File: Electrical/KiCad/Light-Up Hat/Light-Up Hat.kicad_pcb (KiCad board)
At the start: 2 copper layers, 39.9 x 20.1 mm, 18 parts, among them J1 Conn_01x04, Q1 MMBT3906, SW1 SW_SPST, U1 AP1117-33, U2 PIC10F220-IOT

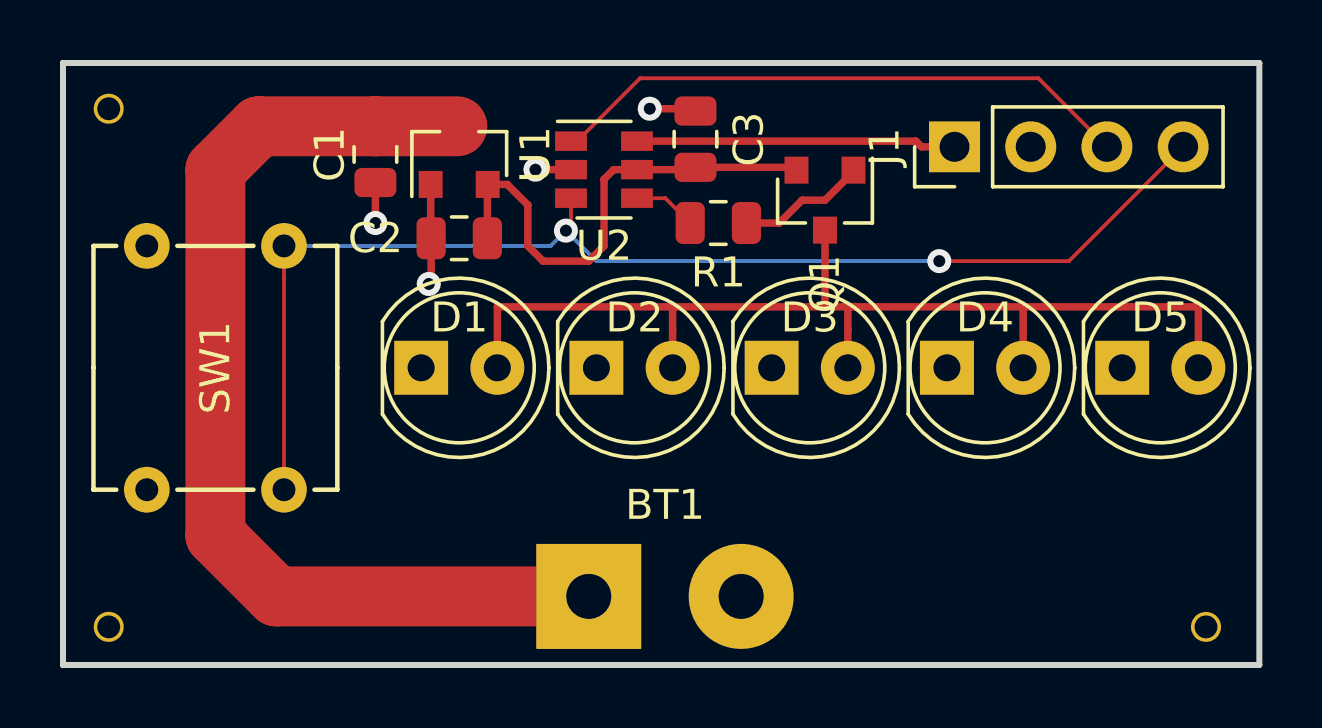
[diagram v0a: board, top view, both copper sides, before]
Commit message: fixed board design for new revision
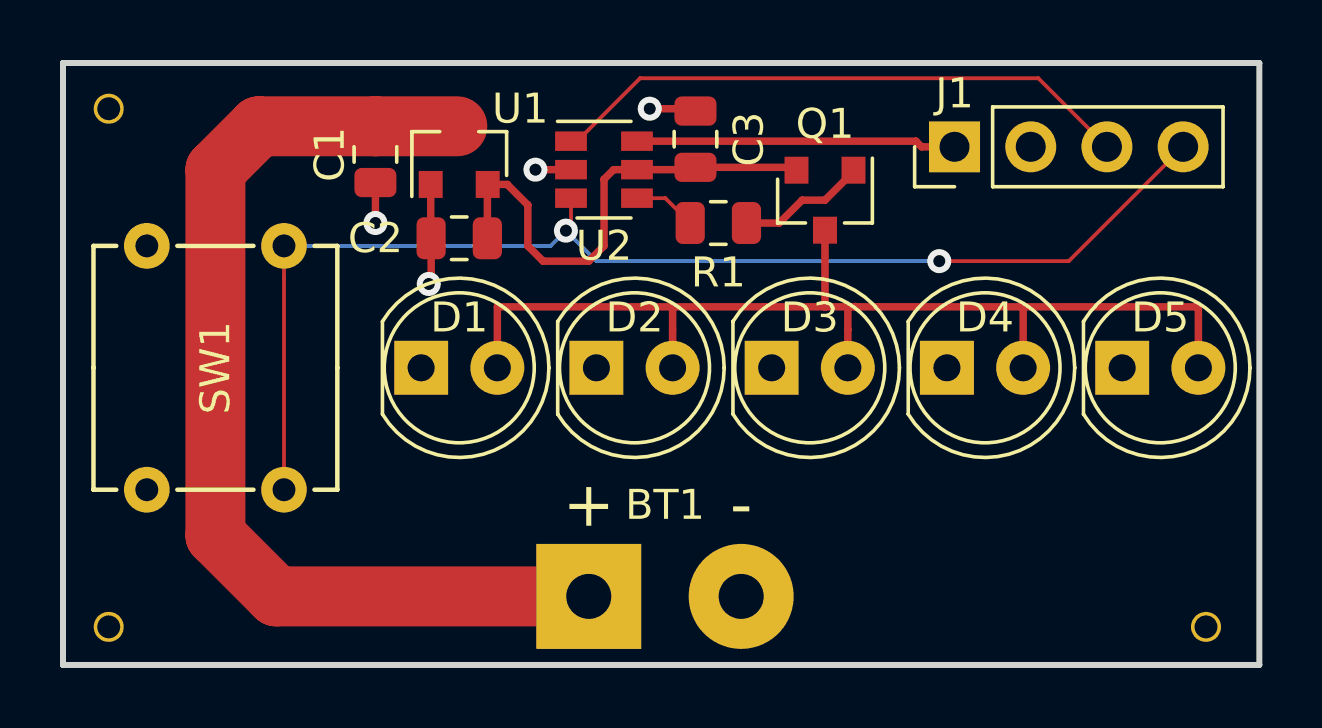
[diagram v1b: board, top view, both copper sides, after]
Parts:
- U1: value AP1117-33 -> XC6206
- U2: value PIC10F220-IOT -> PIC10F200-IOT
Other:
- board text added: "+"
- board text added: "-"
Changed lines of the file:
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@@
   (general
     (thickness 1.6)
-    (drawings 6)
+    (drawings 8)
     (tracks 83)
     (zones 0)
@@
       (creategerberjobfile false)
       (excludeedgelayer false)
-      (linewidth 0.100000)
+      (linewidth 0.150000)
       (plotframeref false)
       (viasonmask false)
@@
     (descr "Through hole straight pin header, 1x04, 2.54mm pitch, single row")
     (tags "Through hole pin header THT 1x04 2.54mm single row")
-    (fp_text reference J1 (at 0 -2.33 90) (layer F.SilkS)
+    (fp_text reference J1 (at 1.778 0 180) (layer F.SilkS)
       (effects (font (size 1 1) (thickness 0.15)))
     )
@@
       (effects (font (size 1 1) (thickness 0.15)))
     )
-    (fp_text value PIC10F220-IOT (at 0 2.9) (layer F.Fab)
+    (fp_text value PIC10F200-IOT (at 0 2.9) (layer F.Fab)
       (effects (font (size 1 1) (thickness 0.15)))
     )
@@
     (tags SOT-23)
     (attr smd)
-    (fp_text reference Q1 (at 2.794 0 270) (layer F.SilkS)
+    (fp_text reference Q1 (at -2.54 0) (layer F.SilkS)
       (effects (font (size 1 1) (thickness 0.15)))
     )
@@
     (tags SOT-23)
     (attr smd)
-    (fp_text reference U1 (at 0 2.54 90) (layer F.SilkS)
-      (effects (font (size 1 1) (thickness 0.15)))
-    )
-    (fp_text value AP1117-33 (at 0 2.5 90) (layer F.Fab)
+    (fp_text reference U1 (at 1.524 2.032 180) (layer F.SilkS)
+      (effects (font (size 1 1) (thickness 0.15)))
+    )
+    (fp_text value XC6206 (at 0 2.5 90) (layer F.Fab)
       (effects (font (size 1 1) (thickness 0.15)))
     )
@@
     )
     (pad "" np_thru_hole circle (at 0 0) (size 1 1) (drill 0.762) (layers *.Cu *.Mask))
+  )
+  (gr_text - (at 147.066 106.172) (layer F.SilkS)
+    (effects (font (size 1.5 1.5) (thickness 0.3)))
+  )
+  (gr_text + (at 141.986 106.172) (layer F.SilkS)
+    (effects (font (size 1.5 1.5) (thickness 0.3)))
   )
   (gr_text "EN-HAT-CED PCB\nREV 1.0" (at 143.5862 104.9782) (layer B.SilkS)
@@
   (segment (start 141.224 97.028) (end 142.24 98.044) (width 0.127) (layer B.Cu) (net 6))
   (segment (start 142.24 98.044) (end 150.114 98.044) (width 0.127) (layer B.Cu) (net 6))
+  (segment (start 150.114 98.044) (end 150.114 98.044) (width 0.127) (layer B.Cu) (net 6))
+  (via (at 153.67 98.044) (size 0.8) (drill 0.4) (layers F.Cu B.Cu) (net 6))
+  (segment (start 150.114 98.044) (end 153.67 98.044) (width 0.127) (layer B.Cu) (net 6))
+  (segment (start 157.988 98.044) (end 153.67 98.044) (width 0.127) (layer F.Cu) (net 6))
+  (segment (start 161.798 94.234) (end 157.988 98.044) (width 0.127) (layer F.Cu) (net 6))
+  (segment (start 144.5385 95.946) (end 143.594 95.946) (width 0.127) (layer F.Cu) (net 7))
+  (segment (start 145.3665 96.774) (end 144.5385 95.946) (width 0.127) (layer F.Cu) (net 7))
   (segment (start 156.464 99.568) (end 156.464 101.6) (width 0.25) (layer F.Cu) (net 8))
   (segment (start 138.938 101.6) (end 138.938 99.568) (width 0.25) (layer F.Cu) (net 8))
@@
   (segment (start 150.86 99.552) (end 150.876 99.568) (width 0.25) (layer F.Cu) (net 8))
   (segment (start 150.622 99.568) (end 150.876 99.568) (width 0.25) (layer F.Cu) (net 8))
-  (segment (start 150.114 98.044) (end 150.114 98.044) (width 0.127) (layer B.Cu) (net 6))
-  (via (at 153.67 98.044) (size 0.8) (drill 0.4) (layers F.Cu B.Cu) (net 6))
-  (segment (start 150.114 98.044) (end 153.67 98.044) (width 0.127) (layer B.Cu) (net 6))
-  (segment (start 157.988 98.044) (end 153.67 98.044) (width 0.127) (layer F.Cu) (net 6))
-  (segment (start 161.798 94.234) (end 157.988 98.044) (width 0.127) (layer F.Cu) (net 6))
-  (segment (start 144.5385 95.946) (end 143.594 95.946) (width 0.127) (layer F.Cu) (net 7))
-  (segment (start 145.3665 96.774) (end 144.5385 95.946) (width 0.127) (layer F.Cu) (net 7))
   (segment (start 144.78 99.568) (end 147.828 99.568) (width 0.25) (layer F.Cu) (net 8))
   (segment (start 147.828 99.568) (end 148.59 99.568) (width 0.25) (layer F.Cu) (net 8))
